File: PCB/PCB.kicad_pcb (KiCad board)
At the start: 2 copper layers, 67 x 73 mm, 10 parts, among them J1 Conn_01x04_Socket, J2 Conn_01x04_Socket, J3 Conn_01x04_Socket, J4 Conn_01x04_Socket, SW1 SW_Push, SW2 SW_Push, SW3 SW_Push, U5 ESP32-DevKitC, U6 SD1306, U7 SD1309

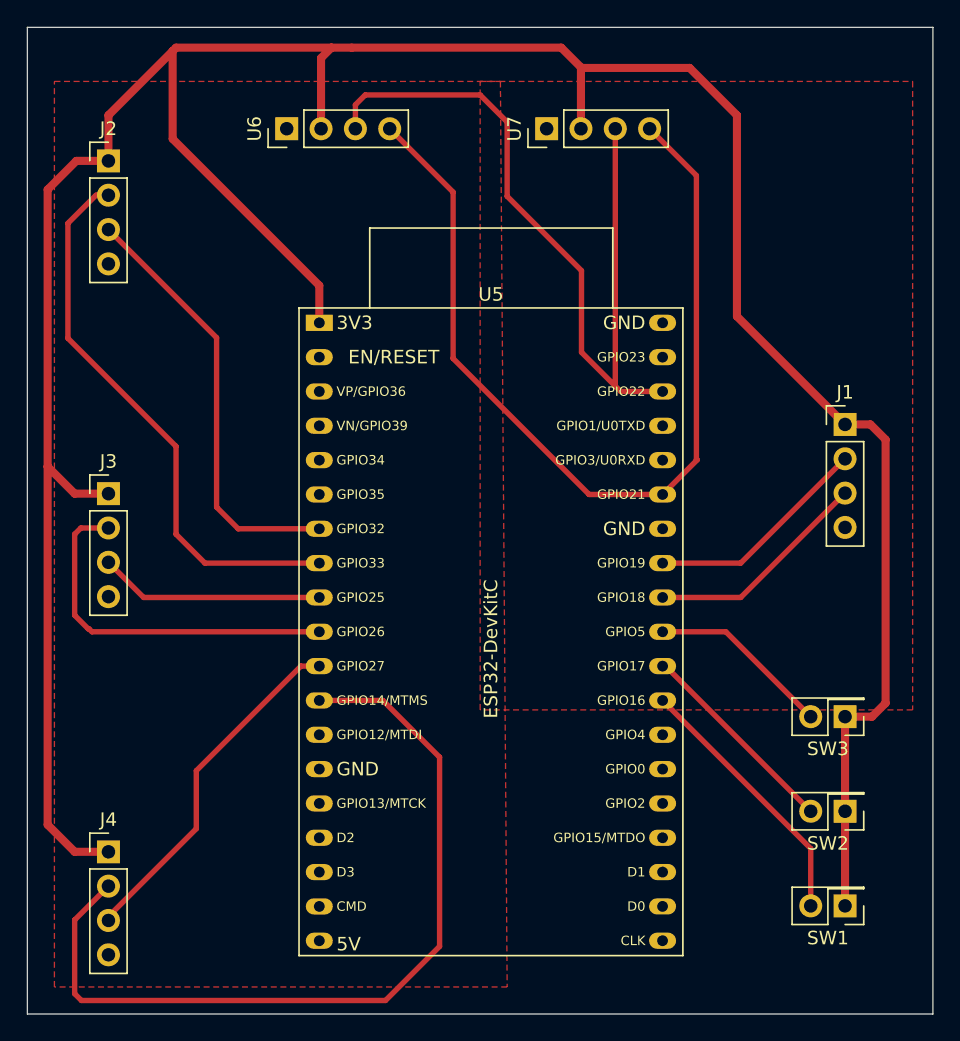
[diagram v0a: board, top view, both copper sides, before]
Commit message: update pcb
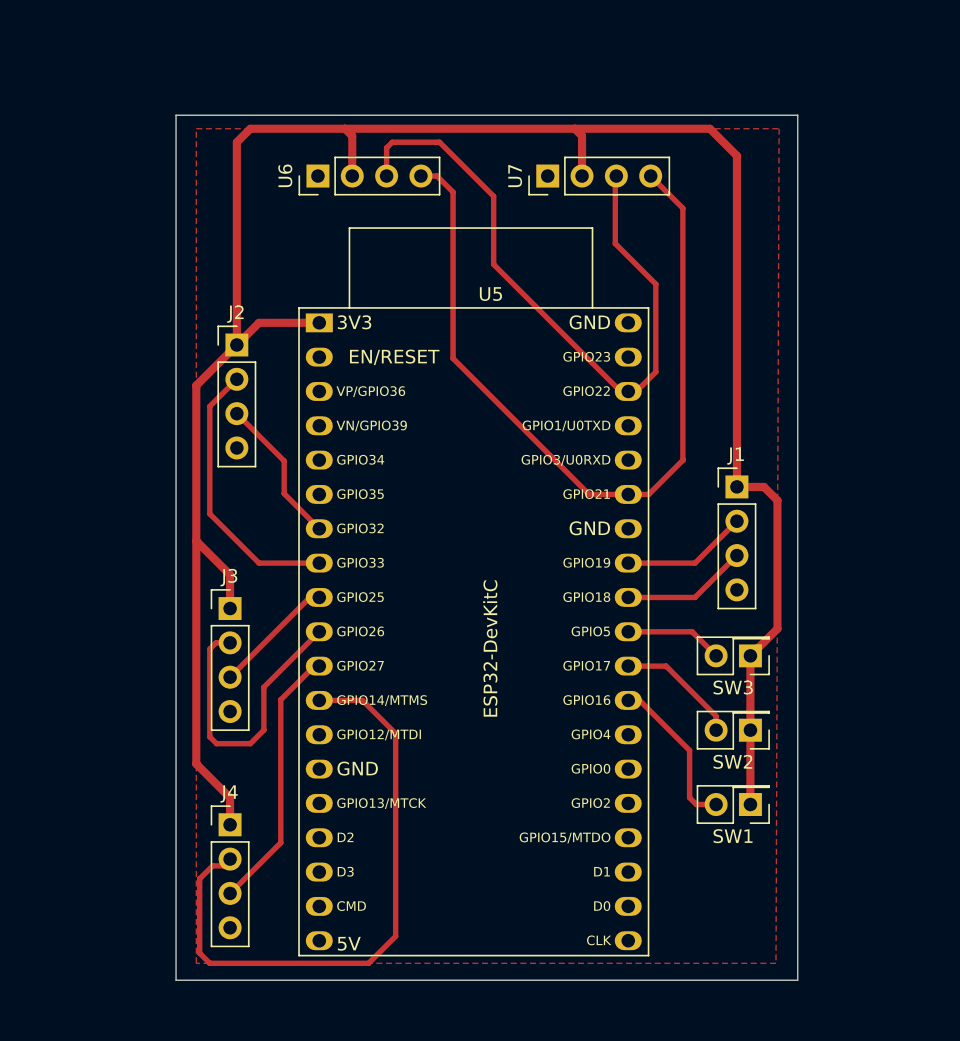
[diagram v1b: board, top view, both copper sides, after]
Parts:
- U5: footprint PCM_Espressif:ESP32-DevKitC -> _custom-footprint:ESP32-DevKitC
- moved J2 16.6 mm to (90.5, 67.0)
- moved J3 12.4 mm to (90.0, 86.5)
- moved SW1 10.3 mm to (128.5, 101.0)
- moved J1 9.24 mm to (127.5, 77.5)
- moved J4 9.22 mm to (90.0, 102.5)
- moved SW2 9.22 mm to (128.5, 95.5)
- moved SW3 8.32 mm to (128.5, 90.0)
- moved U6 4.19 mm to (96.5, 54.5)
- moved U7 3.50 mm to (113.5, 54.5)
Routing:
- net +3.3V: track 219.5 -> 162.6 mm
- net /CLK2: track 41.7 -> 20.4 mm
- net /DATA2: track 32.1 -> 11.0 mm
- net /CLK4: track 62.5 -> 45.7 mm
- net Net-(U5-GPIO22): track 59.7 -> 48.6 mm
- net Net-(U5-GPIO21): track 68.2 -> 59.5 mm
- net /BTN1: track 19.7 -> 11.7 mm
- net /DATA3: track 16.7 -> 9.04 mm
- net /DATA1: track 16.7 -> 9.32 mm
- net /CLK1: track 16.7 -> 9.32 mm
- net /BTN2: track 15.4 -> 9.07 mm
- net /BTN3: track 13.6 -> 7.24 mm
- net /DATA4: track 26.1 -> 19.8 mm
- net /CLK3: track 27.3 -> 21.8 mm
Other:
- board size 67 x 73 mm -> 46 x 64 mm
